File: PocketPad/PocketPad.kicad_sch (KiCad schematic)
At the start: 39 parts, among them SW0 SW_THT_6x6, SW1 SW_THT_6x6, SW10 SW_THT_6x6, SW11 SW_THT_6x6, SW12 SW_THT_6x6, SW13 SW_THT_6x6, SW14 SW_THT_6x6, SW15 SW_THT_6x6, SW16 SW_THT_6x6, SW17 SW_THT_6x6, SW2 SW_THT_6x6, SW3 SW_THT_6x6, SW4 SW_THT_6x6, SW5 SW_THT_6x6, SW6 SW_THT_6x6, SW7 SW_THT_6x6, SW8 SW_THT_6x6, SW9 SW_THT_6x6

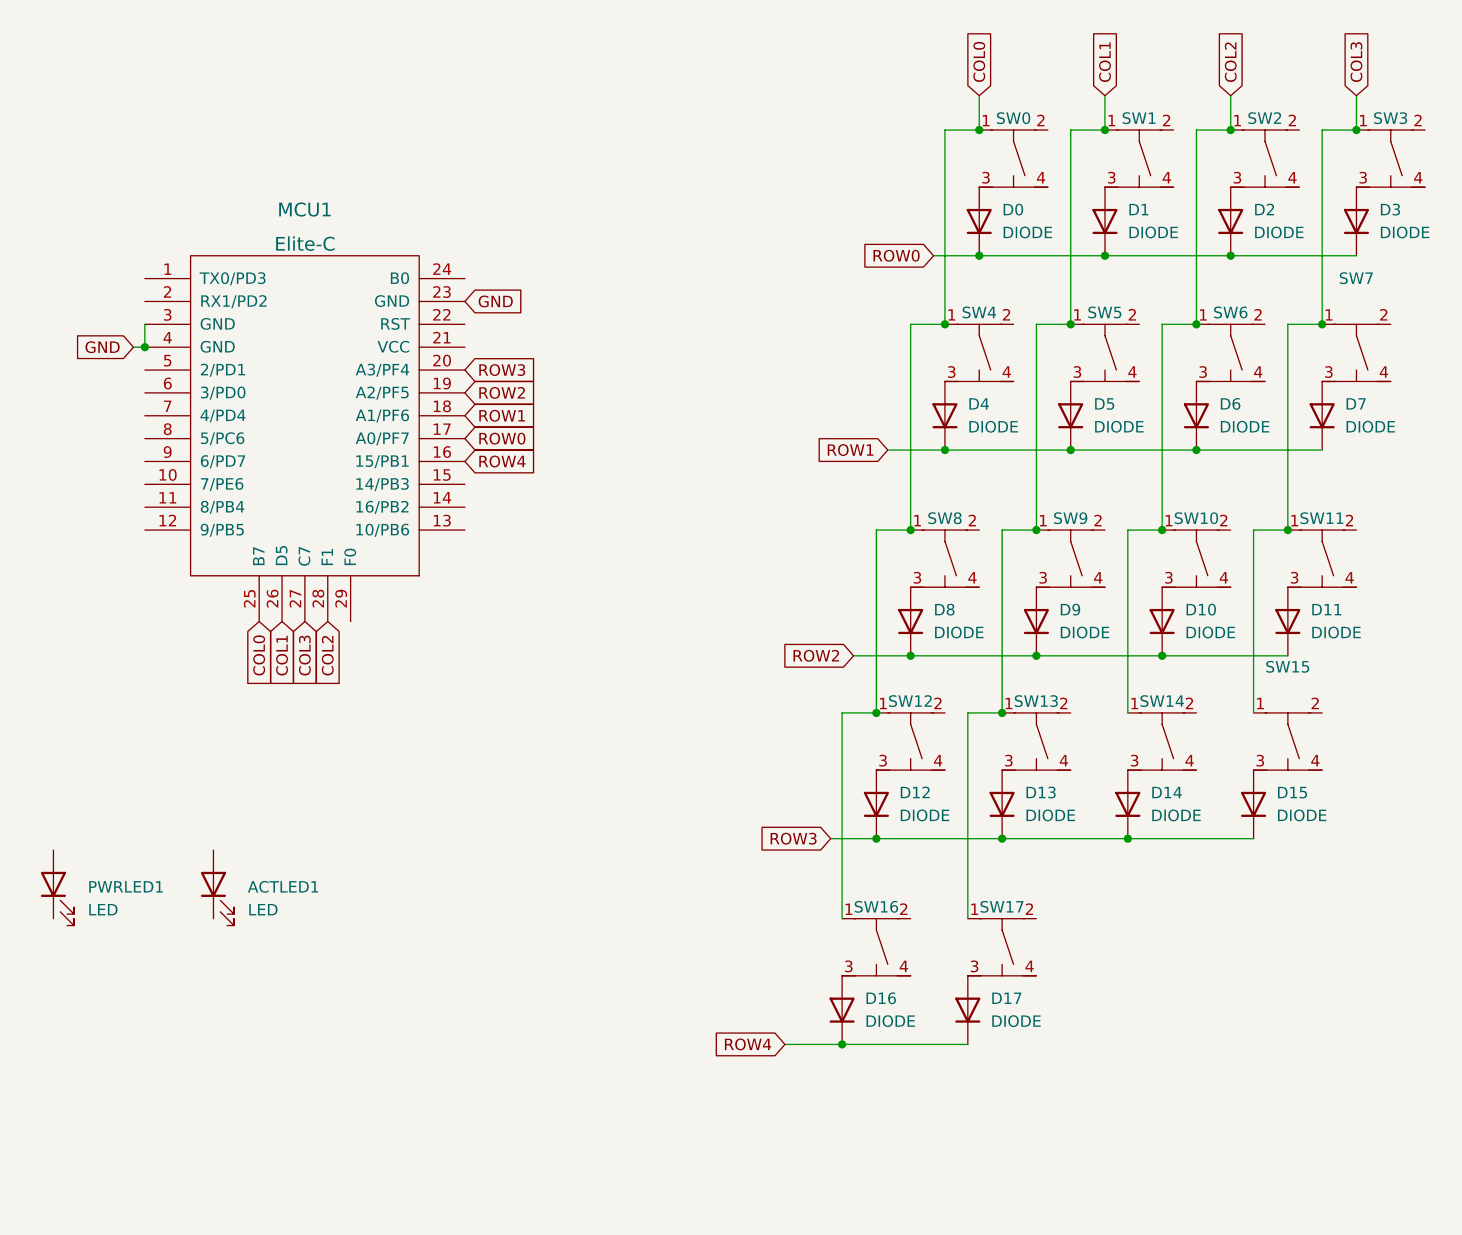
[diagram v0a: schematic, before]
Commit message: V1 complete
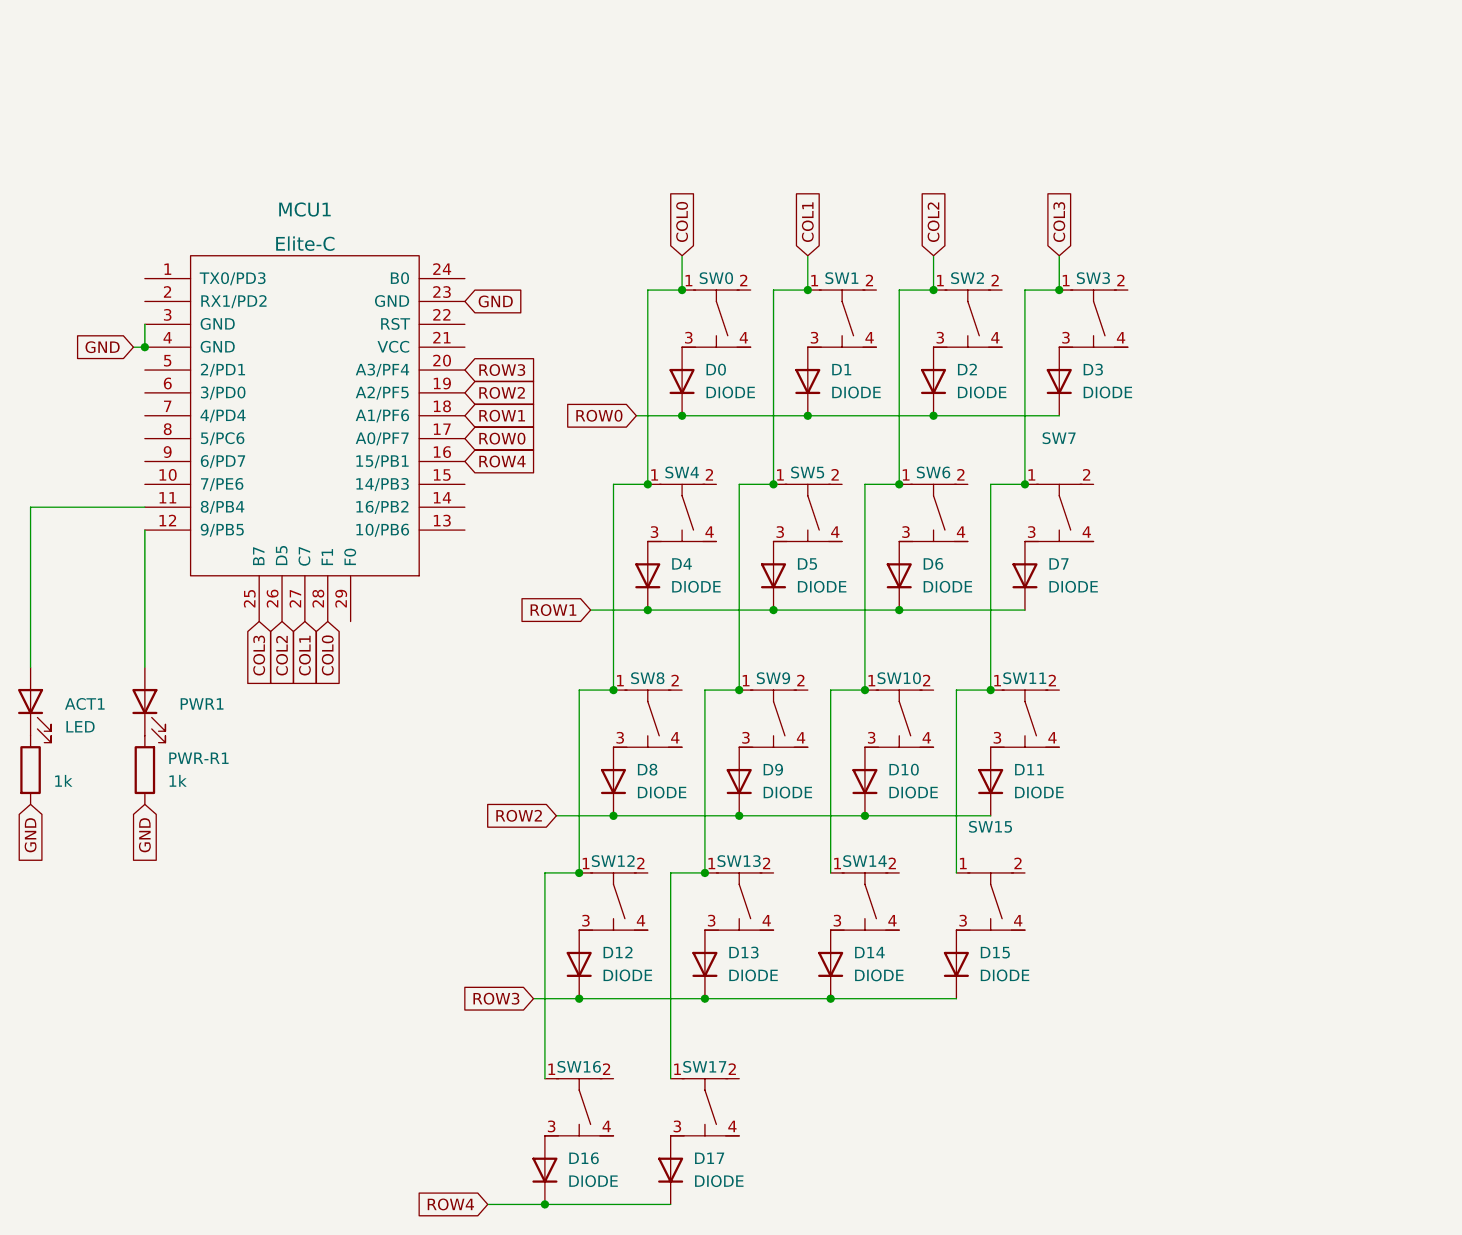
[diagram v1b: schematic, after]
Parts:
- added ACT-R1, PWR-R1: 1k, Resistor_THT:R_Axial_DIN0207_L6.3mm_D2.5mm_P10.16mm_Horizontal, symbol Device:R
- renumbered ACTLED1 to ACT1, PWRLED1 to PWR1
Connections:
- net COL0: now also MCU1.28 (F1); no longer MCU1.25 (B7)
- net COL1: now also MCU1.27 (C7); no longer MCU1.26 (D5)
- net COL2: now also MCU1.26 (D5); no longer MCU1.28 (F1)
- net COL3: now also MCU1.25 (B7); no longer MCU1.27 (C7)
- net GND: now also ACT-R1.2, PWR-R1.1
- net at ACT1.1 (K): now also ACT-R1.1
- net at ACT1.2 (A): now also MCU1.11 (8/PB4)
- net at MCU1.12 (9/PB5): now also PWR1.2 (A)
- net at PWR1.1 (K): now also PWR-R1.2
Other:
- moved on the sheet: ACT1, D0, D1, D10, D11, D12, D13, D14, D15, D16, D17, D2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
